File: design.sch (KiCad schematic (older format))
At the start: 15 parts, among them J1 USB_C_Receptacle, J2 Conn_01x05, Q1 2N7002K, Q2 2N7002K, Q3 2N7002K, U1 ATtiny814-SS

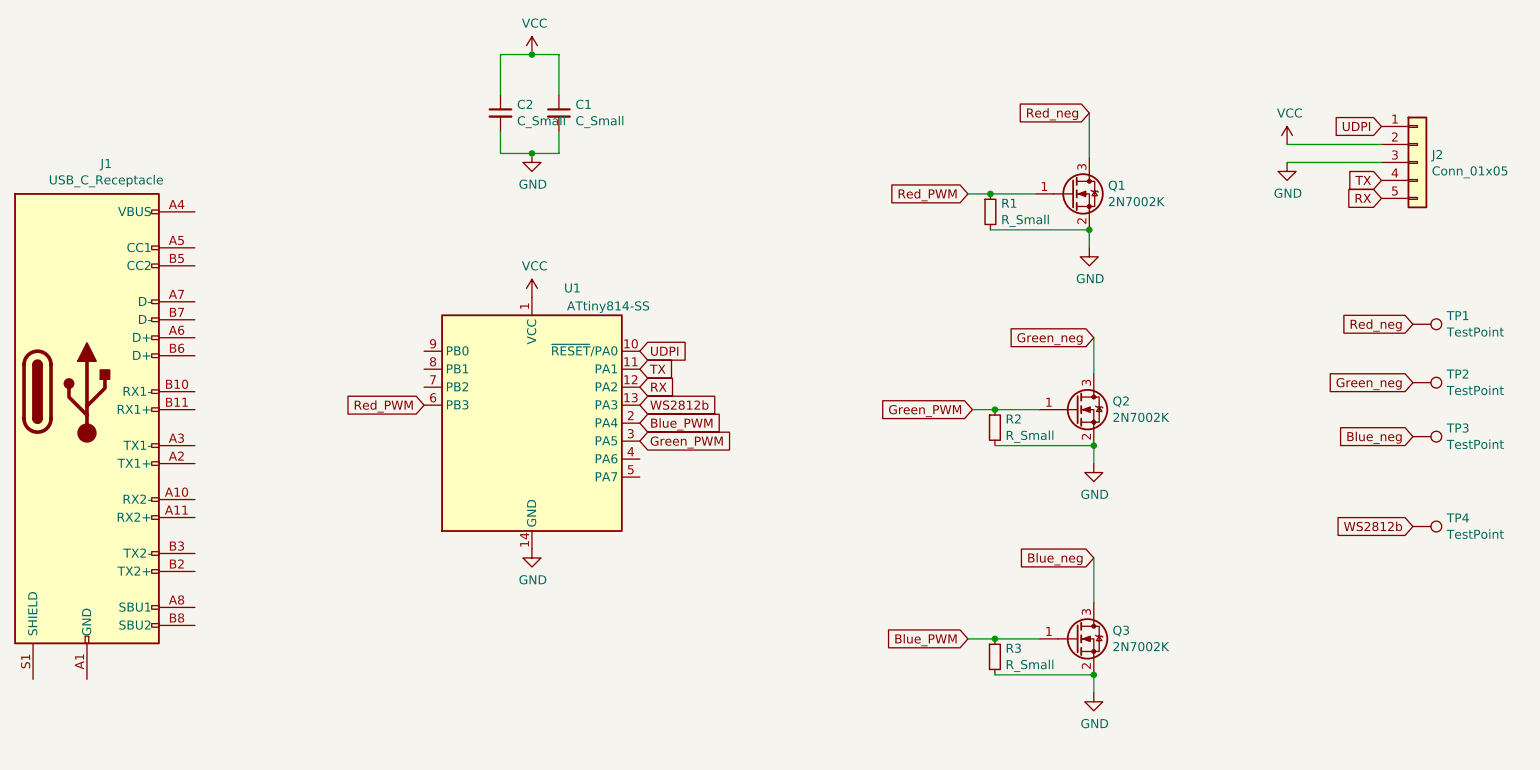
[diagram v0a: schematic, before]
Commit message: add components
usb resistor cc, power flags, mosfet gate resistor
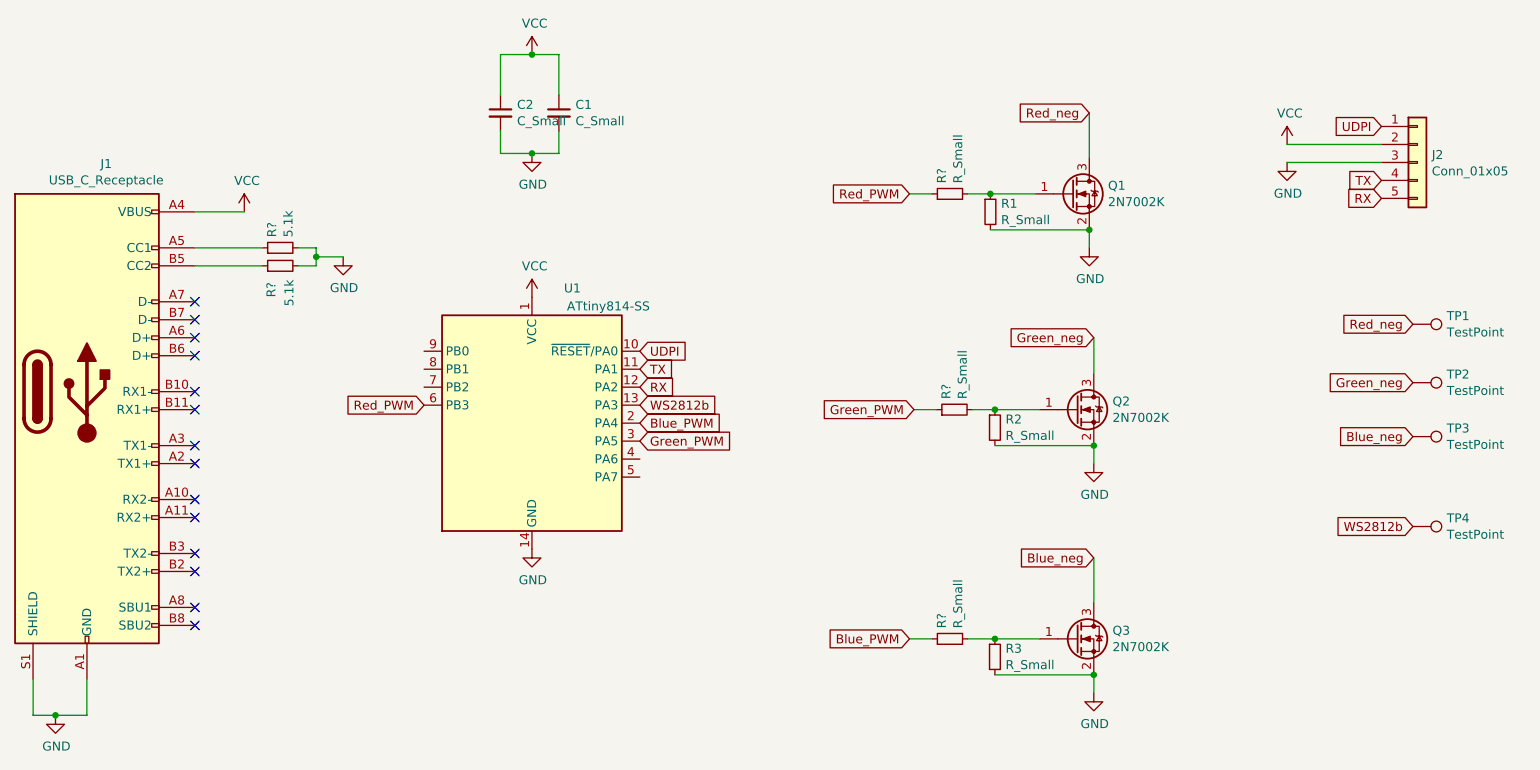
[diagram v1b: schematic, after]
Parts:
- added R? (x3): R_Small, Resistor_SMD:R_0805_2012Metric, symbol Device:R_Small
- added R? (x2): 5.1k, Resistor_SMD:R_0805_2012Metric, symbol Device:R_Small
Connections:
- net Blue_PWM: now also R?.1; no longer Q3.1 (G), R3.1
- net GND: now also J1.A1 (GND), J1.A12 (GND), J1.B1 (GND), J1.B12 (GND), J1.S1 (SHIELD), R?.2, R?.2
- net Green_PWM: now also R?.1; no longer Q2.1 (G), R2.1
- net Red_PWM: now also R?.1; no longer Q1.1 (G), R1.1
- net VCC: now also J1.A4 (VBUS), J1.A9 (VBUS), J1.B4 (VBUS), J1.B9 (VBUS)
- net at J1.A5 (CC1): now also R?.1
- net at J1.B5 (CC2): now also R?.1
- new net: Q1.1 (G), R1.1, R?.2
- new net: Q2.1 (G), R2.1, R?.2
- new net: Q3.1 (G), R3.1, R?.2
- no-connect marks 0 -> 14
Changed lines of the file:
@@
 	7125 2675 7675 2675
 Connection ~ 7675 2675
-Text GLabel 7000 2475 0    50   Input ~ 0
+Text GLabel 6675 2475 0    50   Input ~ 0
 Red_PWM
-Text GLabel 7025 3675 0    50   Input ~ 0
+Text GLabel 6700 3675 0    50   Input ~ 0
 Green_PWM
-Text GLabel 7000 4950 0    50   Input ~ 0
+Text GLabel 6675 4950 0    50   Input ~ 0
 Blue_PWM
 Wire Wire Line
@@
 	4400 1700 4400 1925
 Connection ~ 4575 1700
+$Comp
+L Device:R_Small R?
+U 1 1 61A6A719
+P 6900 2475
+F 0 "R?" H 6959 2521 50  0000 L CNN
+F 1 "R_Small" H 6959 2430 50  0000 L CNN
+F 2 "Resistor_SMD:R_0805_2012Metric" H 6900 2475 50  0001 C CNN
+F 3 "~" H 6900 2475 50  0001 C CNN
+	1    6900 2475
+	0    -1   -1   0
+$EndComp
+Wire Wire Line
+	6675 2475 6800 2475
+$Comp
+L Device:R_Small R?
+U 1 1 61A6CC22
+P 6925 3675
+F 0 "R?" H 6984 3721 50  0000 L CNN
+F 1 "R_Small" H 6984 3630 50  0000 L CNN
+F 2 "Resistor_SMD:R_0805_2012Metric" H 6925 3675 50  0001 C CNN
+F 3 "~" H 6925 3675 50  0001 C CNN
+	1    6925 3675
+	0    -1   -1   0
+$EndComp
+Wire Wire Line
+	6700 3675 6825 3675
+$Comp
+L Device:R_Small R?
+U 1 1 61A6D9D6
+P 6900 4950
+F 0 "R?" H 6959 4996 50  0000 L CNN
+F 1 "R_Small" H 6959 4905 50  0000 L CNN
+F 2 "Resistor_SMD:R_0805_2012Metric" H 6900 4950 50  0001 C CNN
+F 3 "~" H 6900 4950 50  0001 C CNN
+	1    6900 4950
+	0    -1   -1   0
+$EndComp
+Wire Wire Line
+	6675 4950 6800 4950
+NoConn ~ 2700 3075
+NoConn ~ 2700 3175
+NoConn ~ 2700 3275
+NoConn ~ 2700 3375
+NoConn ~ 2700 3575
+NoConn ~ 2700 3675
+NoConn ~ 2700 3875
+NoConn ~ 2700 3975
+NoConn ~ 2700 4175
+NoConn ~ 2700 4275
+NoConn ~ 2700 4475
+NoConn ~ 2700 4575
+NoConn ~ 2700 4775
+NoConn ~ 2700 4875
+$Comp
+L power:GND #PWR?
+U 1 1 61A7334E
+P 1925 5375
+F 0 "#PWR?" H 1925 5125 50  0001 C CNN
+F 1 "GND" H 1930 5202 50  0000 C CNN
+F 2 "" H 1925 5375 50  0001 C CNN
+F 3 "" H 1925 5375 50  0001 C CNN
+	1    1925 5375
+	1    0    0    -1
+$EndComp
+Wire Wire Line
+	1925 5375 1800 5375
+Wire Wire Line
+	1800 5375 1800 5175
+Wire Wire Line
+	1925 5375 2100 5375
+Wire Wire Line
+	2100 5375 2100 5175
+Connection ~ 1925 5375
+$Comp
+L power:VCC #PWR?
+U 1 1 61A74E6E
+P 2975 2575
+F 0 "#PWR?" H 2975 2425 50  0001 C CNN
+F 1 "VCC" H 2990 2748 50  0000 C CNN
+F 2 "" H 2975 2575 50  0001 C CNN
+F 3 "" H 2975 2575 50  0001 C CNN
+	1    2975 2575
+	1    0    0    -1
+$EndComp
+Wire Wire Line
+	2975 2575 2700 2575
+$Comp
+L Device:R_Small R?
+U 1 1 61A75EA7
+P 3175 2775
+F 0 "R?" H 3234 2821 50  0000 L CNN
+F 1 "5.1k" H 3234 2730 50  0000 L CNN
+F 2 "Resistor_SMD:R_0805_2012Metric" H 3175 2775 50  0001 C CNN
+F 3 "~" H 3175 2775 50  0001 C CNN
+	1    3175 2775
+	0    -1   -1   0
+$EndComp
+Wire Wire Line
+	3075 2775 2700 2775
+Wire Wire Line
+	2700 2875 3075 2875
+$Comp
+L Device:R_Small R?
+U 1 1 61A77F57
+P 3175 2875
+F 0 "R?" H 3000 2925 50  0000 L CNN
+F 1 "5.1k" H 2950 2825 50  0000 L CNN
+F 2 "Resistor_SMD:R_0805_2012Metric" H 3175 2875 50  0001 C CNN
+F 3 "~" H 3175 2875 50  0001 C CNN
+	1    3175 2875
+	0    -1   -1   0
+$EndComp
+$Comp
+L power:GND #PWR?
+U 1 1 61A78369
+P 3525 2825
+F 0 "#PWR?" H 3525 2575 50  0001 C CNN
+F 1 "GND" H 3530 2652 50  0000 C CNN
+F 2 "" H 3525 2825 50  0001 C CNN
+F 3 "" H 3525 2825 50  0001 C CNN
+	1    3525 2825
+	1    0    0    -1
+$EndComp
+Wire Wire Line
+	3275 2875 3375 2875
+Wire Wire Line
+	3375 2875 3375 2825
+Wire Wire Line
+	3375 2825 3525 2825
+Wire Wire Line
+	3375 2825 3375 2775
+Wire Wire Line
+	3375 2775 3275 2775
+Connection ~ 3375 2825
 $EndSCHEMATC

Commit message: Revert "add components"
This reverts commit 60fcf040a8541399063354e6f95bf0141af0d636.
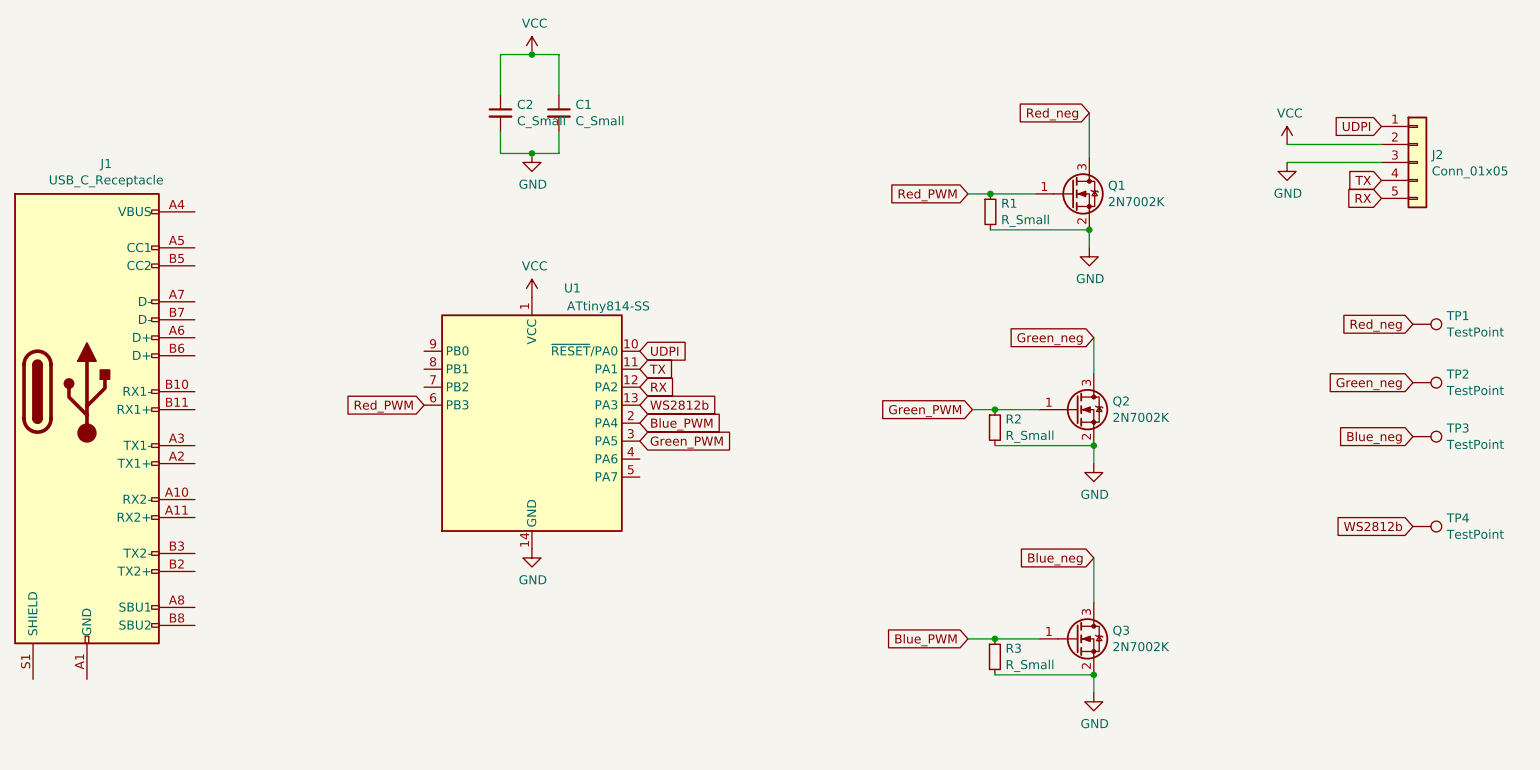
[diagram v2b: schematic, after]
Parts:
- removed R? (x3): R_Small, Resistor_SMD:R_0805_2012Metric, symbol Device:R_Small
- removed R? (x2): 5.1k, Resistor_SMD:R_0805_2012Metric, symbol Device:R_Small
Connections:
- net Blue_PWM: now also Q3.1 (G), R3.1
- net GND: no longer J1.A1 (GND), J1.A12 (GND), J1.B1 (GND), J1.B12 (GND), J1.S1 (SHIELD)
- net Green_PWM: now also Q2.1 (G), R2.1
- net Red_PWM: now also Q1.1 (G), R1.1
- net VCC: no longer J1.A4 (VBUS), J1.A9 (VBUS), J1.B4 (VBUS), J1.B9 (VBUS)
- new net: J1.A1 (GND), J1.A12 (GND), J1.B1 (GND), J1.B12 (GND)
- new net: J1.A4 (VBUS), J1.A9 (VBUS), J1.B4 (VBUS), J1.B9 (VBUS)
- no-connect marks 14 -> 0
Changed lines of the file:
@@
 	7125 2675 7675 2675
 Connection ~ 7675 2675
-Text GLabel 6675 2475 0    50   Input ~ 0
+Text GLabel 7000 2475 0    50   Input ~ 0
 Red_PWM
-Text GLabel 6700 3675 0    50   Input ~ 0
+Text GLabel 7025 3675 0    50   Input ~ 0
 Green_PWM
-Text GLabel 6675 4950 0    50   Input ~ 0
+Text GLabel 7000 4950 0    50   Input ~ 0
 Blue_PWM
 Wire Wire Line
@@
 	4400 1700 4400 1925
 Connection ~ 4575 1700
-$Comp
-L Device:R_Small R?
-U 1 1 61A6A719
-P 6900 2475
-F 0 "R?" H 6959 2521 50  0000 L CNN
-F 1 "R_Small" H 6959 2430 50  0000 L CNN
-F 2 "Resistor_SMD:R_0805_2012Metric" H 6900 2475 50  0001 C CNN
-F 3 "~" H 6900 2475 50  0001 C CNN
-	1    6900 2475
-	0    -1   -1   0
-$EndComp
-Wire Wire Line
-	6675 2475 6800 2475
-$Comp
-L Device:R_Small R?
-U 1 1 61A6CC22
-P 6925 3675
-F 0 "R?" H 6984 3721 50  0000 L CNN
-F 1 "R_Small" H 6984 3630 50  0000 L CNN
-F 2 "Resistor_SMD:R_0805_2012Metric" H 6925 3675 50  0001 C CNN
-F 3 "~" H 6925 3675 50  0001 C CNN
-	1    6925 3675
-	0    -1   -1   0
-$EndComp
-Wire Wire Line
-	6700 3675 6825 3675
-$Comp
-L Device:R_Small R?
-U 1 1 61A6D9D6
-P 6900 4950
-F 0 "R?" H 6959 4996 50  0000 L CNN
-F 1 "R_Small" H 6959 4905 50  0000 L CNN
-F 2 "Resistor_SMD:R_0805_2012Metric" H 6900 4950 50  0001 C CNN
-F 3 "~" H 6900 4950 50  0001 C CNN
-	1    6900 4950
-	0    -1   -1   0
-$EndComp
-Wire Wire Line
-	6675 4950 6800 4950
-NoConn ~ 2700 3075
-NoConn ~ 2700 3175
-NoConn ~ 2700 3275
-NoConn ~ 2700 3375
-NoConn ~ 2700 3575
-NoConn ~ 2700 3675
-NoConn ~ 2700 3875
-NoConn ~ 2700 3975
-NoConn ~ 2700 4175
-NoConn ~ 2700 4275
-NoConn ~ 2700 4475
-NoConn ~ 2700 4575
-NoConn ~ 2700 4775
-NoConn ~ 2700 4875
-$Comp
-L power:GND #PWR?
-U 1 1 61A7334E
-P 1925 5375
-F 0 "#PWR?" H 1925 5125 50  0001 C CNN
-F 1 "GND" H 1930 5202 50  0000 C CNN
-F 2 "" H 1925 5375 50  0001 C CNN
-F 3 "" H 1925 5375 50  0001 C CNN
-	1    1925 5375
-	1    0    0    -1
-$EndComp
-Wire Wire Line
-	1925 5375 1800 5375
-Wire Wire Line
-	1800 5375 1800 5175
-Wire Wire Line
-	1925 5375 2100 5375
-Wire Wire Line
-	2100 5375 2100 5175
-Connection ~ 1925 5375
-$Comp
-L power:VCC #PWR?
-U 1 1 61A74E6E
-P 2975 2575
-F 0 "#PWR?" H 2975 2425 50  0001 C CNN
-F 1 "VCC" H 2990 2748 50  0000 C CNN
-F 2 "" H 2975 2575 50  0001 C CNN
-F 3 "" H 2975 2575 50  0001 C CNN
-	1    2975 2575
-	1    0    0    -1
-$EndComp
-Wire Wire Line
-	2975 2575 2700 2575
-$Comp
-L Device:R_Small R?
-U 1 1 61A75EA7
-P 3175 2775
-F 0 "R?" H 3234 2821 50  0000 L CNN
-F 1 "5.1k" H 3234 2730 50  0000 L CNN
-F 2 "Resistor_SMD:R_0805_2012Metric" H 3175 2775 50  0001 C CNN
-F 3 "~" H 3175 2775 50  0001 C CNN
-	1    3175 2775
-	0    -1   -1   0
-$EndComp
-Wire Wire Line
-	3075 2775 2700 2775
-Wire Wire Line
-	2700 2875 3075 2875
-$Comp
-L Device:R_Small R?
-U 1 1 61A77F57
-P 3175 2875
-F 0 "R?" H 3000 2925 50  0000 L CNN
-F 1 "5.1k" H 2950 2825 50  0000 L CNN
-F 2 "Resistor_SMD:R_0805_2012Metric" H 3175 2875 50  0001 C CNN
-F 3 "~" H 3175 2875 50  0001 C CNN
-	1    3175 2875
-	0    -1   -1   0
-$EndComp
-$Comp
-L power:GND #PWR?
-U 1 1 61A78369
-P 3525 2825
-F 0 "#PWR?" H 3525 2575 50  0001 C CNN
-F 1 "GND" H 3530 2652 50  0000 C CNN
-F 2 "" H 3525 2825 50  0001 C CNN
-F 3 "" H 3525 2825 50  0001 C CNN
-	1    3525 2825
-	1    0    0    -1
-$EndComp
-Wire Wire Line
-	3275 2875 3375 2875
-Wire Wire Line
-	3375 2875 3375 2825
-Wire Wire Line
-	3375 2825 3525 2825
-Wire Wire Line
-	3375 2825 3375 2775
-Wire Wire Line
-	3375 2775 3275 2775
-Connection ~ 3375 2825
 $EndSCHEMATC
